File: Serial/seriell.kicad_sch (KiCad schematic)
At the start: 27 parts, among them J1 Conn_01x10_Pin, J10 Conn_01x06, J11 Conn_01x06, J12 TTL, J13 Conn_01x10_Pin, J14 Conn_01x10_Pin, J15 Conn_01x10_Pin, J16 Conn_01x10_Pin, J17 Conn_01x10_Pin, J18 Conn_01x10_Pin, J19 Bluetooth, J2 Conn_01x10_Pin, J20 Conn_01x04, J3 Conn_01x10_Pin, J30 Flash, J4 Conn_01x10_Pin, J5 Conn_01x10_Pin, J6 Conn_01x10_Pin, J7 Conn_02x04_Counter_Clockwise, J8 BT

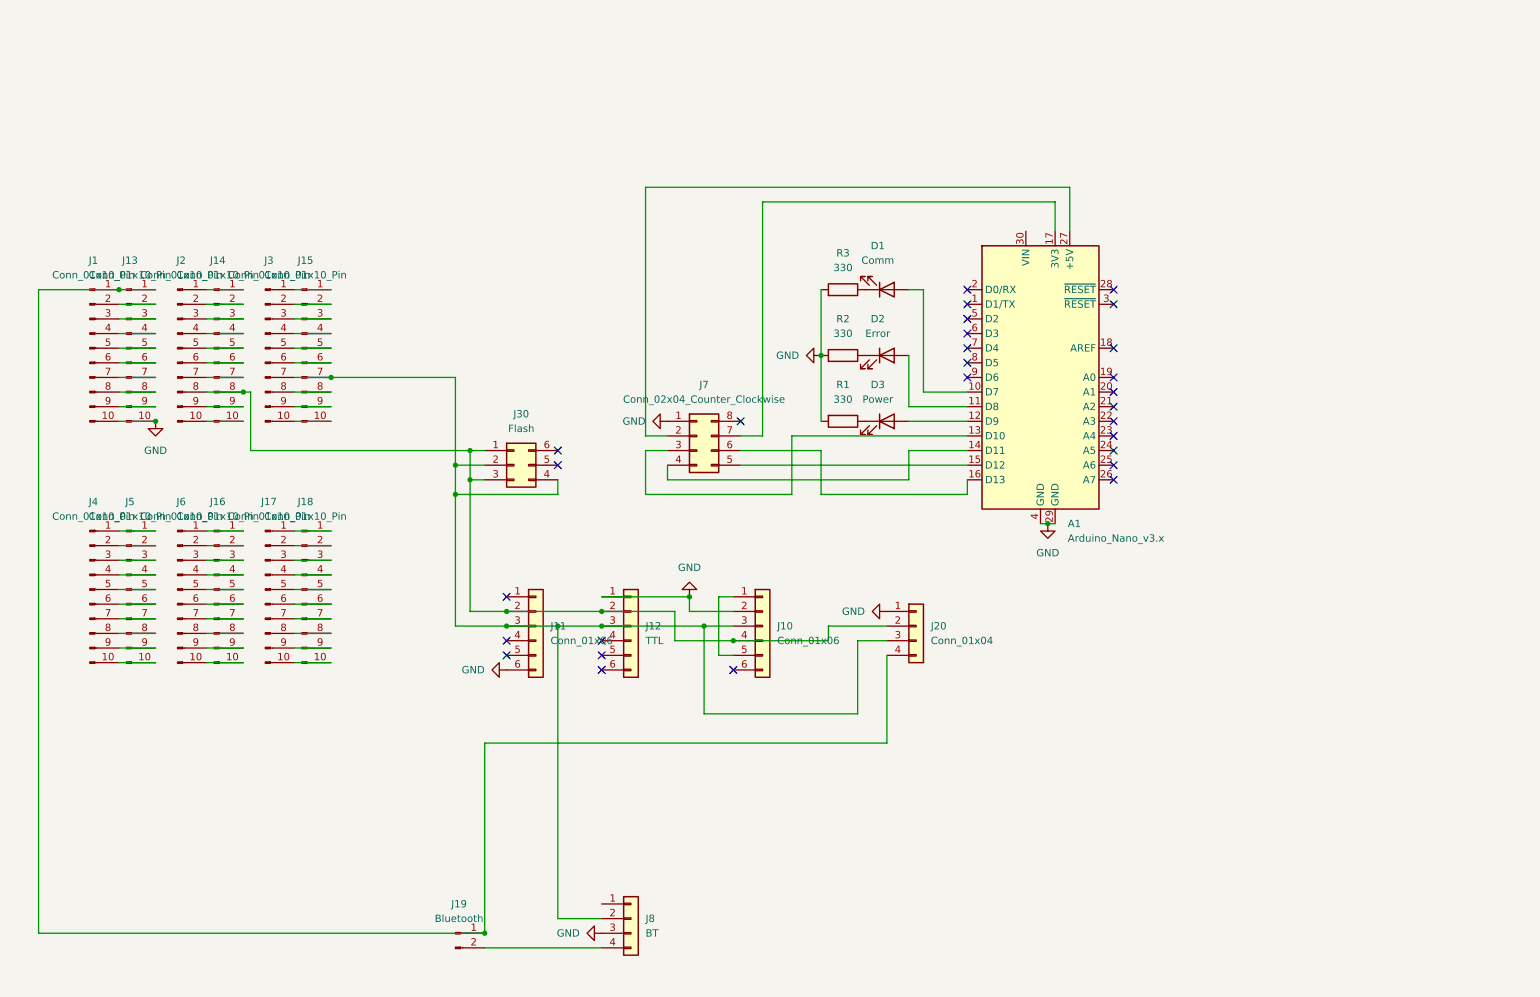
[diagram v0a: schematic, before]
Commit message: serial redesign
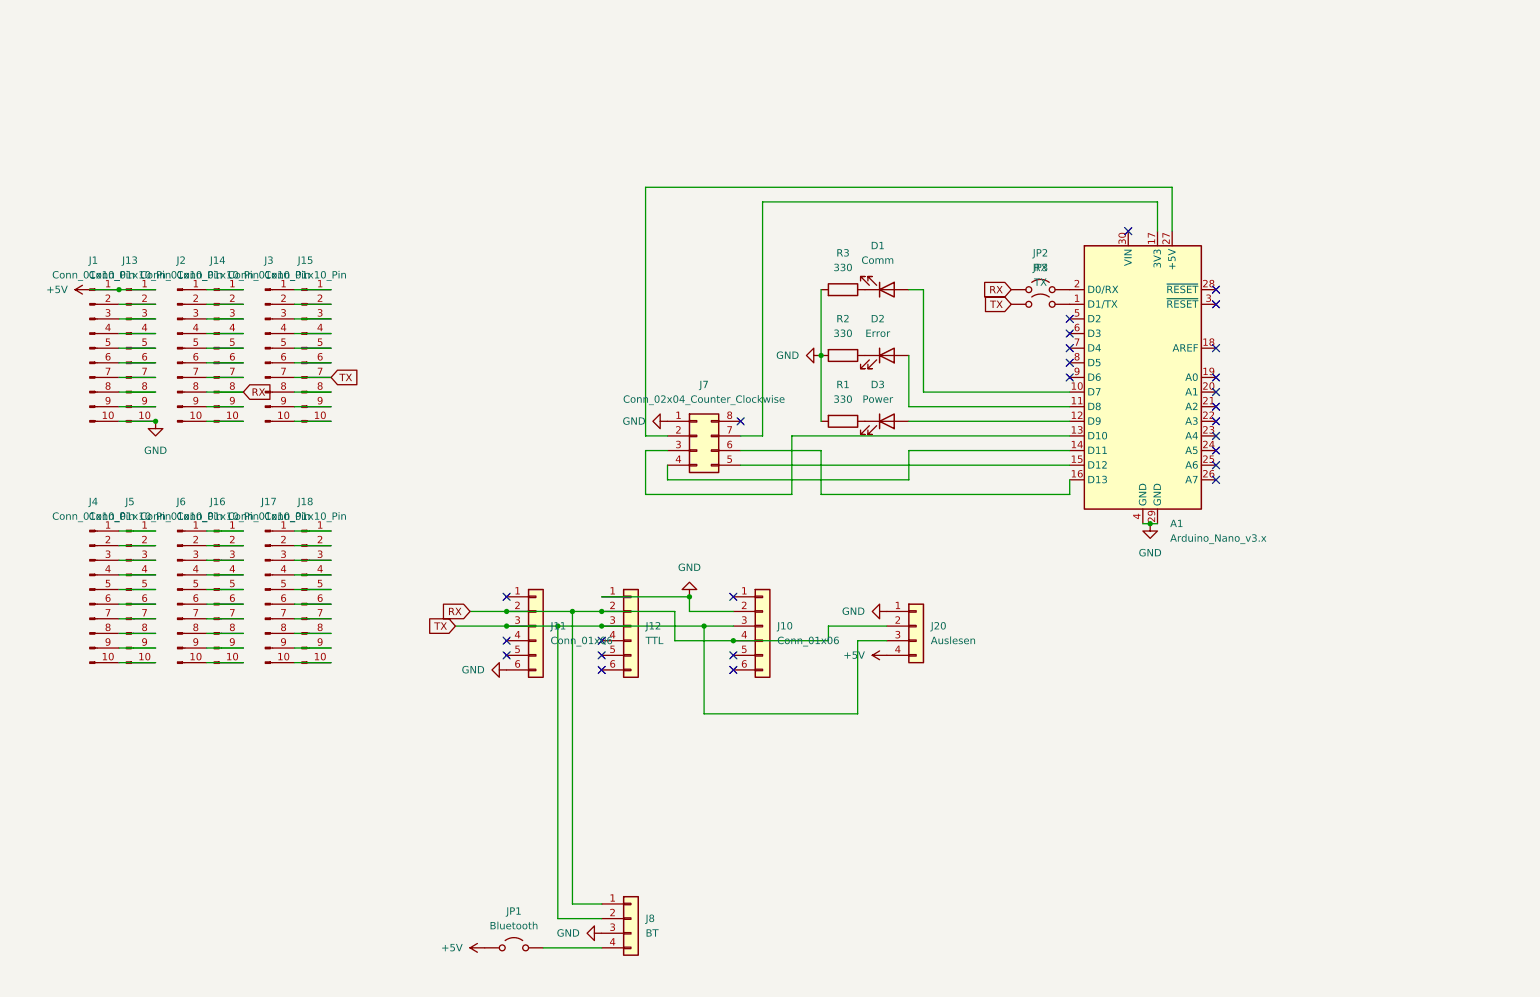
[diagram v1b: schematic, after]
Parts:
- removed J19: Bluetooth, Connector_PinHeader_2.54mm:PinHeader_1x02_P2.54mm_Vertical, symbol Connector:Conn_01x02_Pin
- removed J30: Flash, Connector_PinHeader_2.54mm:PinHeader_2x03_P2.54mm_Vertical, symbol Connector_Generic:Conn_02x03_Counter_Clockwise
- added JP1: Bluetooth, Jumper:SolderJumper-2_P1.3mm_Open_Pad1.0x1.5mm, symbol Jumper:Jumper_2_Open
- added JP2: RX, Jumper:SolderJumper-2_P1.3mm_Open_Pad1.0x1.5mm, symbol Jumper:Jumper_2_Open
- added JP3: TX, Jumper:SolderJumper-2_P1.3mm_Open_Pad1.0x1.5mm, symbol Jumper:Jumper_2_Open
- J20: value Conn_01x04 -> Auslesen
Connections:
- net TX: now reaches J10.3 (Pin_3), J11.3 (Pin_3), J12.3 (Pin_3), J15.7 (Pin_7), J20.3 (Pin_3), J3.7 (Pin_7), J8.2 (Pin_2)
- net TX: now also JP3.1 (A)
- net RX: now reaches J10.4 (Pin_4), J11.2 (Pin_2), J12.2 (Pin_2), J14.8 (Pin_8), J2.8 (Pin_8), J20.2 (Pin_2)
- net RX: now also J8.1 (Pin_1), JP2.1 (A)
- net at J10.1 (Pin_1): no longer J10.5 (Pin_5)
- net +5V: now reaches J1.1 (Pin_1), J13.1 (Pin_1), J20.4 (Pin_4)
- net +5V: now also JP1.1 (A)
- net at J8.4 (Pin_4): now also JP1.2 (B)
- net at A1.1 (D1/TX): now also JP3.2 (B)
- net at A1.2 (D0/RX): now also JP2.2 (B)
- no-connect marks 28 -> 27
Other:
- moved on the sheet: A1

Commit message: wemos
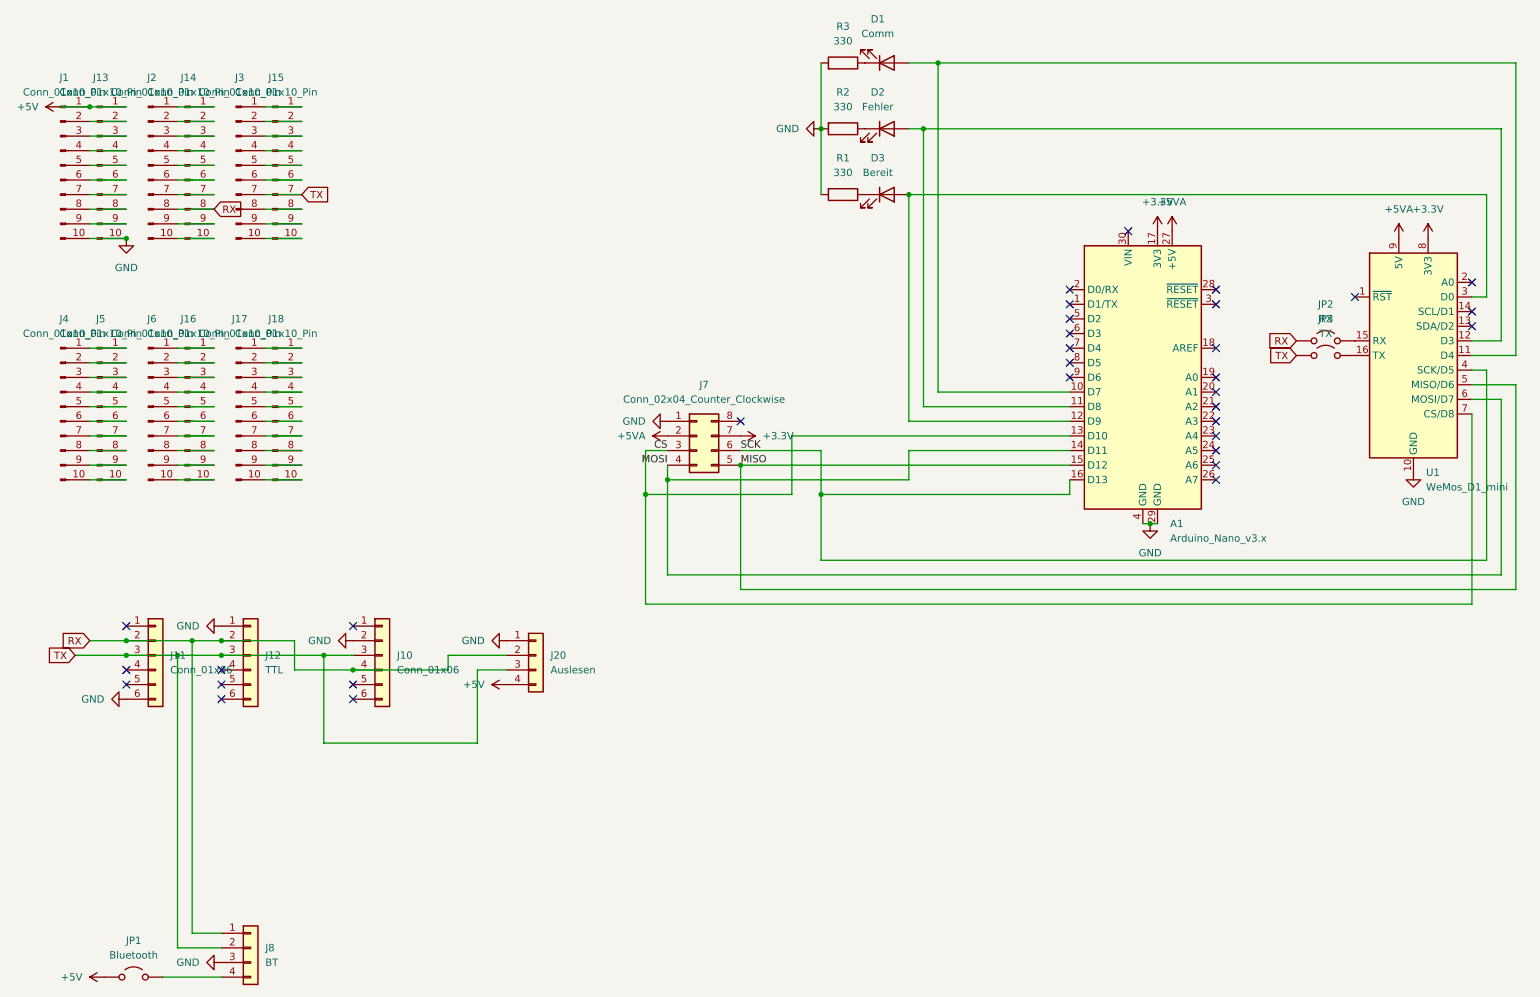
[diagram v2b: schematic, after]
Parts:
- added U1: WeMos_D1_mini, Module:WEMOS_D1_mini_light, symbol MCU_Module:WeMos_D1_mini
- D2: value Error -> Fehler
- D3: value Power -> Bereit
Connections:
- net GND: now also U1.10 (GND)
- net at A1.12 (D9), D3.2 (A): now also U1.3 (D0)
- net at JP3.2 (B): now also U1.16 (TX); no longer A1.1 (D1/TX)
- net at JP2.2 (B): now also U1.15 (RX); no longer A1.2 (D0/RX)
- net at A1.11 (D8), D2.2 (A): now also U1.12 (D3)
- net at A1.10 (D7), D1.2 (A): now also U1.11 (D4)
- net CS: now reaches A1.13 (D10), J7.3 (Pin_3)
- net CS: now also U1.7 (CS/D8)
- net MOSI: now reaches A1.14 (D11), J7.4 (Pin_4)
- net MOSI: now also U1.6 (MOSI/D7)
- net MISO: now reaches A1.15 (D12), J7.5 (Pin_5)
- net MISO: now also U1.5 (MISO/D6)
- net SCK: now reaches A1.16 (D13), J7.6 (Pin_6)
- net SCK: now also U1.4 (SCK/D5)
- net +3.3V: now reaches A1.17 (3V3), J7.7 (Pin_7)
- net +3.3V: now also U1.8 (3V3)
- net +5VA: now reaches A1.27 (+5V), J7.2 (Pin_2)
- net +5VA: now also U1.9 (5V)
- no-connect marks 27 -> 33
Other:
- moved on the sheet: D1, D2, D3, J1, J10, J11, J12, J13, J14, J15, J16, J17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

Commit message: esp
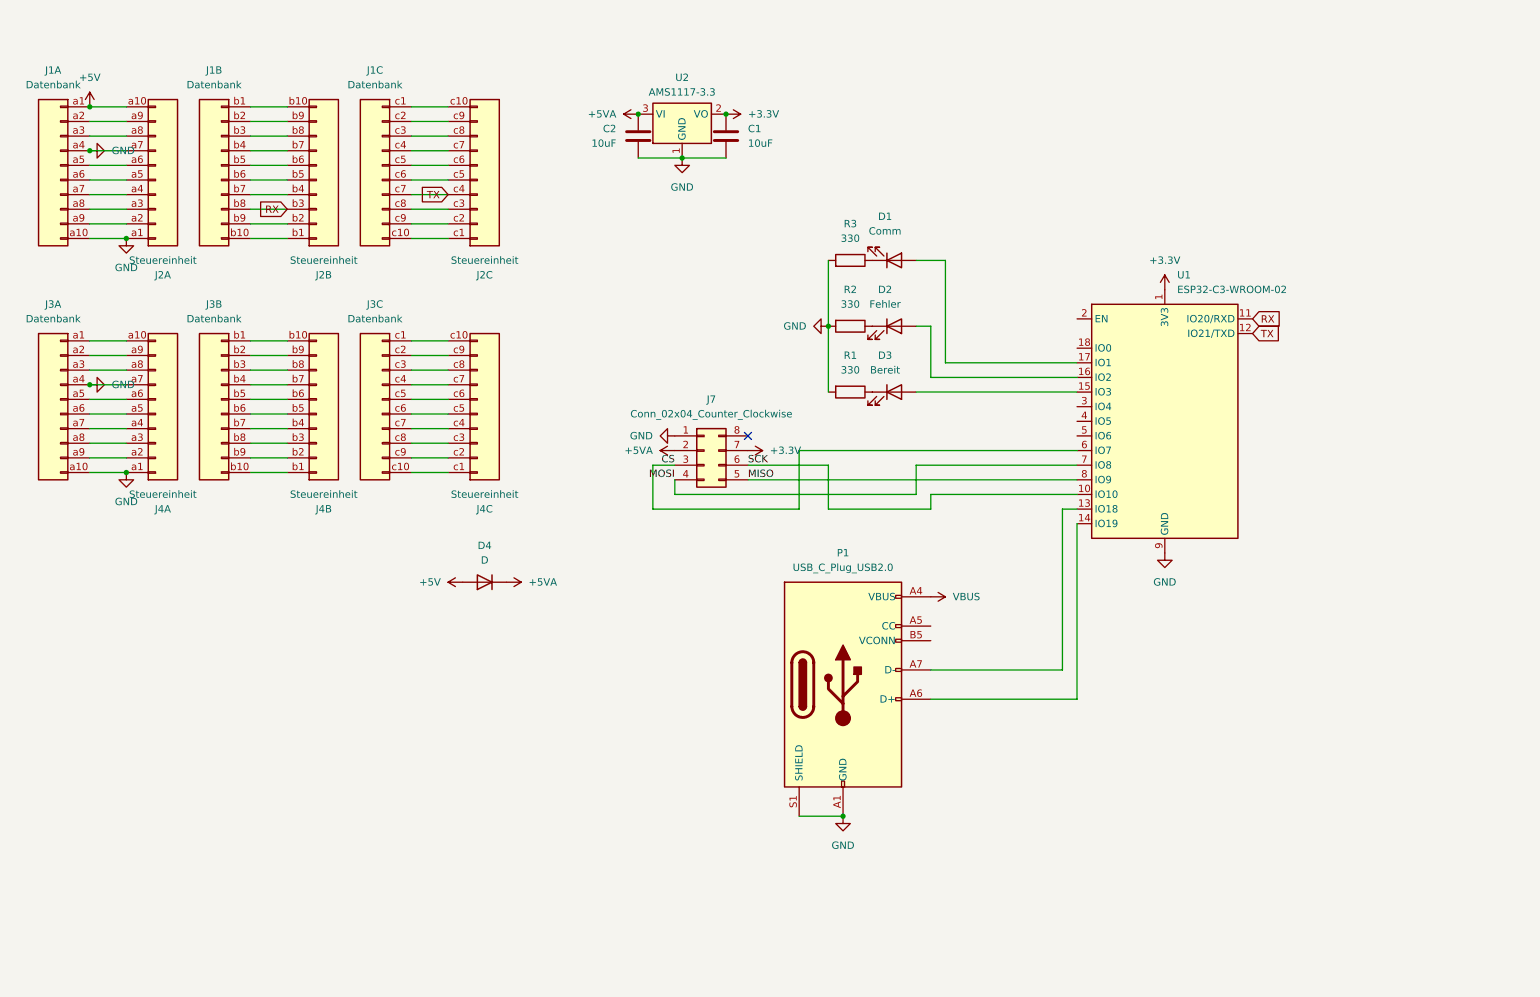
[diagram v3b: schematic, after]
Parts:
- removed A1: Arduino_Nano_v3.x, Module:Arduino_Nano, symbol MCU_Module:Arduino_Nano_v3.x
- removed J1, J13, J14, J15, J16, J17, J18, J2, J3, J4, J5, J6: Conn_01x10_Pin, Connector_PinSocket_2.54mm:PinSocket_1x10_P2.54mm_Vertical, symbol Connector:Conn_01x10_Pin
- removed J10, J11: Conn_01x06, Connector_PinHeader_2.54mm:PinHeader_1x06_P2.54mm_Vertical, symbol Connector_Generic:Conn_01x06
- removed J12: TTL, Connector_PinHeader_2.54mm:PinHeader_1x06_P2.54mm_Vertical, symbol Connector_Generic:Conn_01x06
- removed J20: Auslesen, Connector_PinHeader_2.54mm:PinHeader_1x04_P2.54mm_Vertical, symbol Connector_Generic:Conn_01x04
- removed J8: BT, Connector_PinHeader_2.54mm:PinHeader_1x04_P2.54mm_Vertical, symbol Connector_Generic:Conn_01x04
- removed JP1: Bluetooth, Jumper:SolderJumper-2_P1.3mm_Open_Pad1.0x1.5mm, symbol Jumper:Jumper_2_Open
- removed JP2: RX, Jumper:SolderJumper-2_P1.3mm_Open_Pad1.0x1.5mm, symbol Jumper:Jumper_2_Open
- removed JP3: TX, Jumper:SolderJumper-2_P1.3mm_Open_Pad1.0x1.5mm, symbol Jumper:Jumper_2_Open
- removed U1: WeMos_D1_mini, Module:WEMOS_D1_mini_light, symbol MCU_Module:WeMos_D1_mini
- added C1, C2: 10uF, Capacitor_SMD:C_0603_1608Metric, symbol Device:C
- added D4: D, Diode_SMD:D_SOD-123, symbol Device:D
- added J1, J3: Datenbank, Connector_DIN:DIN41612_C3_3x10_Female_Vertical_THT, symbol DIN41612:DIN41612_03x10_ABC
- added J2, J4: Steuereinheit, Connector_DIN:DIN41612_R3_3x10_Male_Vertical_THT, symbol DIN41612:DIN41612_03x10_ABC
- added P1: USB_C_Plug_USB2.0, Connector_USB:USB_C_Receptacle_G-Switch_GT-USB-7010ASV, symbol Connector:USB_C_Plug_USB2.0
- added U1: ESP32-C3-WROOM-02, RF_Module:ESP32-C3-WROOM-02, symbol RF_Module:ESP32-C3-WROOM-02
- added U2: AMS1117-3.3, Package_TO_SOT_SMD:SOT-223-3_TabPin2, symbol Regulator_Linear:AMS1117-3.3
- D1, D2, D3: footprint LED_THT:LED_D5.0mm -> LED_SMD:LED_0603_1608Metric
- J7: footprint Connector_PinHeader_2.54mm:PinHeader_2x04_P2.54mm_Vertical -> Connector_IDC:IDC-Header_2x04_P2.54mm_Vertical
- R1, R2, R3: footprint Resistor_SMD:R_0805_2012Metric -> LED_SMD:LED_0603_1608Metric
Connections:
- net +3.3V: now also C1.1, U1.1 (3V3), U2.2 (VO)
- net +5V: now also D4.2 (A), J1.a1 (Pin_a1), J2.a10 (Pin_a10)
- net +5VA: now also C2.1, D4.1 (K), U2.3 (VI)
- net CS: now also U1.6 (IO7)
- net GND: now also C1.2, C2.2, J1.a10 (Pin_a10), J1.a4 (Pin_a4), J2.a1 (Pin_a1), J2.a7 (Pin_a7), J3.a10 (Pin_a10), J3.a4 (Pin_a4), J4.a1 (Pin_a1), J4.a7 (Pin_a7), P1.A1 (GND), P1.A12 (GND), P1.B1 (GND), P1.B12 (GND), P1.S1 (SHIELD), U1.19 (GND), U1.9 (GND), U2.1 (GND)
- net MISO: now also U1.8 (IO9)
- net MOSI: now also U1.7 (IO8)
- net RX: now also J1.b8 (Pin_b8), J2.b3 (Pin_b3), U1.11 (IO20/RXD)
- net SCK: now also U1.10 (IO10)
- net TX: now also J1.c7 (Pin_c7), J2.c4 (Pin_c4), U1.12 (IO21/TXD)
- net at D3.2 (A): now also U1.15 (IO3)
- net at D2.2 (A): now also U1.16 (IO2)
- net at D1.2 (A): now also U1.17 (IO1)
- new net: J1.c10 (Pin_c10), J2.c1 (Pin_c1)
- new net: J1.c1 (Pin_c1), J2.c10 (Pin_c10)
- new net: J1.c9 (Pin_c9), J2.c2 (Pin_c2)
- new net: J1.c8 (Pin_c8), J2.c3 (Pin_c3)
- new net: J1.c6 (Pin_c6), J2.c5 (Pin_c5)
- new net: J1.c5 (Pin_c5), J2.c6 (Pin_c6)
- new net: J1.c4 (Pin_c4), J2.c7 (Pin_c7)
- new net: J1.c3 (Pin_c3), J2.c8 (Pin_c8)
- new net: J1.c2 (Pin_c2), J2.c9 (Pin_c9)
- new net: J3.a1 (Pin_a1), J4.a10 (Pin_a10)
- new net: J3.a9 (Pin_a9), J4.a2 (Pin_a2)
- new net: J3.a8 (Pin_a8), J4.a3 (Pin_a3)
- new net: J3.a7 (Pin_a7), J4.a4 (Pin_a4)
- new net: J3.a6 (Pin_a6), J4.a5 (Pin_a5)
- new net: J3.a5 (Pin_a5), J4.a6 (Pin_a6)
- new net: J3.a3 (Pin_a3), J4.a8 (Pin_a8)
- new net: J3.a2 (Pin_a2), J4.a9 (Pin_a9)
- new net: J3.c1 (Pin_c1), J4.c10 (Pin_c10)
- new net: J3.c10 (Pin_c10), J4.c1 (Pin_c1)
- new net: J3.c2 (Pin_c2), J4.c9 (Pin_c9)
- new net: J3.c3 (Pin_c3), J4.c8 (Pin_c8)
- new net: J3.c4 (Pin_c4), J4.c7 (Pin_c7)
- new net: J3.c5 (Pin_c5), J4.c6 (Pin_c6)
- new net: J3.c6 (Pin_c6), J4.c5 (Pin_c5)
- new net: J3.c7 (Pin_c7), J4.c4 (Pin_c4)
- new net: J3.c8 (Pin_c8), J4.c3 (Pin_c3)
- new net: J3.c9 (Pin_c9), J4.c2 (Pin_c2)
- new net: J1.b10 (Pin_b10), J2.b1 (Pin_b1)
- new net: J1.b1 (Pin_b1), J2.b10 (Pin_b10)
- new net: J1.b9 (Pin_b9), J2.b2 (Pin_b2)
- new net: J1.b7 (Pin_b7), J2.b4 (Pin_b4)
- new net: J1.b6 (Pin_b6), J2.b5 (Pin_b5)
- new net: J1.b5 (Pin_b5), J2.b6 (Pin_b6)
- new net: J1.b4 (Pin_b4), J2.b7 (Pin_b7)
- new net: J1.b3 (Pin_b3), J2.b8 (Pin_b8)
- new net: J1.b2 (Pin_b2), J2.b9 (Pin_b9)
- new net: J3.b1 (Pin_b1), J4.b10 (Pin_b10)
- new net: J3.b10 (Pin_b10), J4.b1 (Pin_b1)
- new net: J3.b2 (Pin_b2), J4.b9 (Pin_b9)
- new net: J3.b3 (Pin_b3), J4.b8 (Pin_b8)
- new net: J3.b4 (Pin_b4), J4.b7 (Pin_b7)
- new net: J3.b5 (Pin_b5), J4.b6 (Pin_b6)
- new net: J3.b6 (Pin_b6), J4.b5 (Pin_b5)
- new net: J3.b7 (Pin_b7), J4.b4 (Pin_b4)
- new net: J3.b8 (Pin_b8), J4.b3 (Pin_b3)
- new net: J3.b9 (Pin_b9), J4.b2 (Pin_b2)
- new net: P1.A7 (D-), U1.13 (IO18)
- new net: P1.A6 (D+), U1.14 (IO19)
- new net: J1.a9 (Pin_a9), J2.a2 (Pin_a2)
- new net: J1.a8 (Pin_a8), J2.a3 (Pin_a3)
- new net: J1.a7 (Pin_a7), J2.a4 (Pin_a4)
- new net: J1.a6 (Pin_a6), J2.a5 (Pin_a5)
- new net: J1.a5 (Pin_a5), J2.a6 (Pin_a6)
- new net: J1.a3 (Pin_a3), J2.a8 (Pin_a8)
- new net: J1.a2 (Pin_a2), J2.a9 (Pin_a9)
- new net VBUS: P1.A4 (VBUS), P1.A9 (VBUS), P1.B4 (VBUS), P1.B9 (VBUS)
- no-connect marks 33 -> 1
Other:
- moved on the sheet: D1, D2, D3, J7, R1, R2, R3
